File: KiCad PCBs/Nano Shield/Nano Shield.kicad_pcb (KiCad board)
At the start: 2 copper layers, 72.4 x 35.6 mm, 32 parts, among them J1 Conn_01x15_Female, J10 Screw_Terminal_01x02, J11 Screw_Terminal_01x02, J12 Screw_Terminal_01x02, J13 Screw_Terminal_01x02, J15 Screw_Terminal_01x02, J17 Screw_Terminal_01x02, J18 Screw_Terminal_01x02, J2 Conn_01x15_Female, J3 Screw_Terminal_01x02, J4 Screw_Terminal_01x02, J5 Screw_Terminal_01x02, J6 Screw_Terminal_01x02, J7 Screw_Terminal_01x02, J8 Screw_Terminal_01x02, J9 Screw_Terminal_01x02, SW1 SW_DIP_x02, SW2 SW_DIP_x02, U1 MAX487ESA+T, U2 AMS1117-5.0, U3 ULN2003A

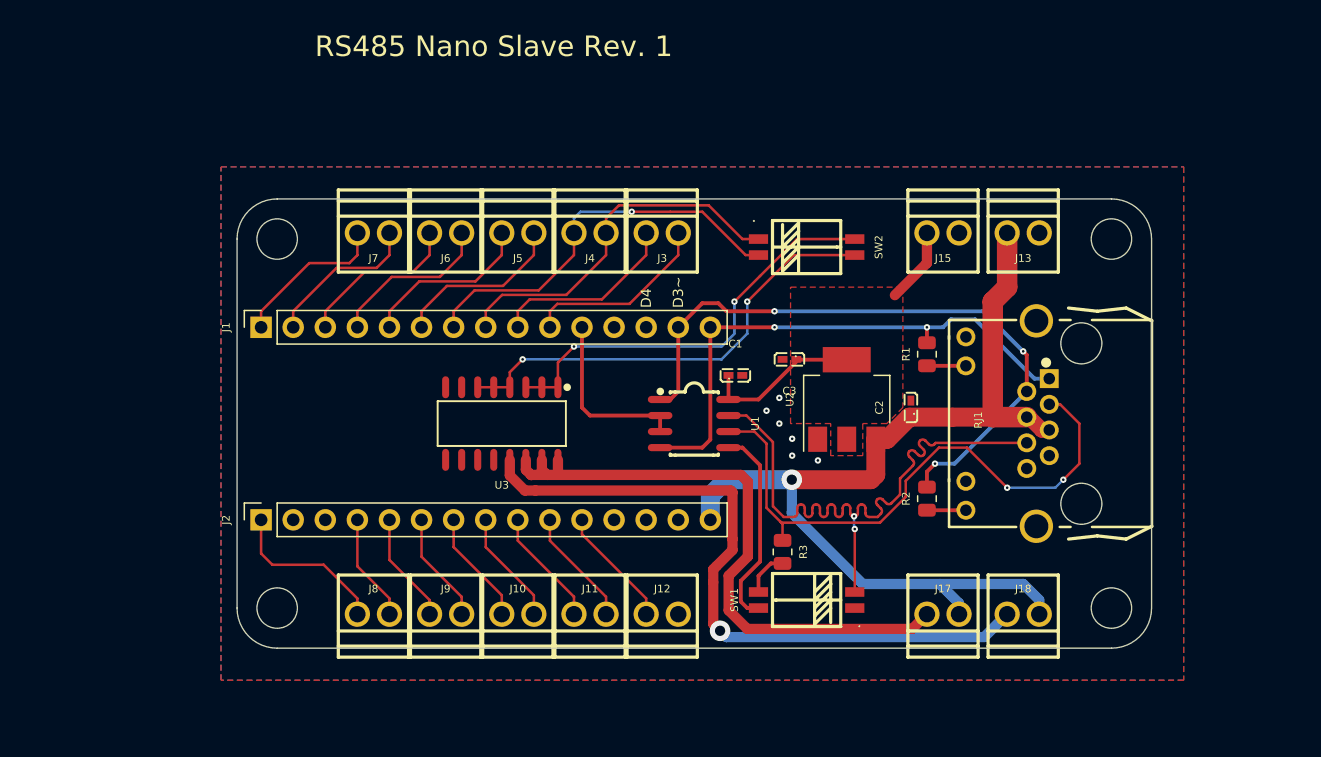
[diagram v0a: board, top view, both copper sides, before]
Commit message: Finished Nano Shield
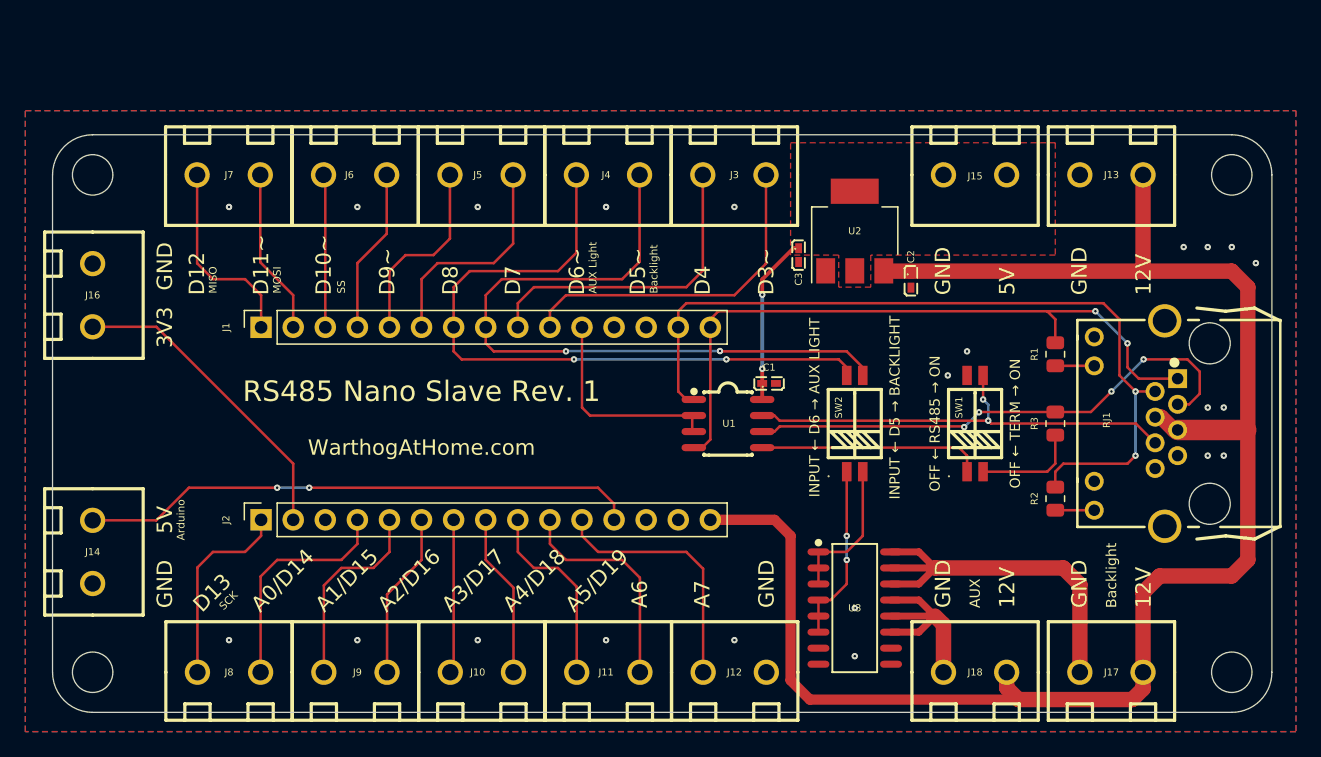
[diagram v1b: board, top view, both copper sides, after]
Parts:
- added J14: Screw_Terminal_01x02, A10 KiCad Libraries:CONN-TH_WJ126V-5.0-2P, F.Cu at (121.9, 111.8)
- added J16: Screw_Terminal_01x02, A10 KiCad Libraries:CONN-TH_WJ126V-5.0-2P, F.Cu at (121.9, 91.4)
- J10, J11, J12, J13, J15, J17, J18, J3, J4, J5, J6, J7, J8, J9: footprint A10 KiCad Libraries:CONN-TH_XY308-2.54-2P -> A10 KiCad Libraries:CONN-TH_WJ126V-5.0-2P
- moved U3 31.5 mm to (182.2, 116.2), turned to -90 degrees
- moved R3 23.9 mm to (198.1, 101.6)
- moved SW1 19.3 mm to (191.8, 101.6), turned to 0 degrees
- moved H1 15.5 mm to (121.9, 81.9)
- moved H3 15.5 mm to (121.9, 121.3)
- moved SW2 14.5 mm to (182.2, 101.6), turned to 0 degrees
- moved J17 14.1 mm to (202.6, 121.3), turned to 90 degrees
- moved U2 13.4 mm to (182.2, 86.4)
- moved J7 12.3 mm to (132.7, 81.9), turned to -90 degrees
- moved J8 12.3 mm to (132.7, 121.3), turned to 90 degrees
- moved H2 10.8 mm to (212.1, 81.9)
- moved H4 10.8 mm to (212.1, 121.3)
- moved R1 10.2 mm to (198.1, 96.1)
- moved R2 10.2 mm to (198.1, 107.5)
- moved RJ1 10.2 mm to (207.9, 101.6)
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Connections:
- J10 pad 1: A4/D18 -> A3/D17
- J10 pad 2: A3/D17 -> A4/D18
- J11 pad 1: A6 -> A5/D19
- J11 pad 2: A5/D19 -> A6
- J12 pad 1: GND -> A7
- J12 pad 2: A7 -> GND
- J17 pad 1: +12V -> BACKLIGHT_GND
- J17 pad 2: BACKLIGHT_GND -> +12V
- J18 pad 1: +12V -> AUX_GND
- J18 pad 2: AUX_GND -> +12V
- J3 pad 1: D4 -> D3~
- J3 pad 2: D3~ -> D4
- J4 pad 1: D6~/AUX_LIGHT -> D5~/BACKLIGHT
- J4 pad 2: D5~/BACKLIGHT -> D6~/AUX_LIGHT
- J5 pad 1: D8 -> D7
- J5 pad 2: D7 -> D8
- J6 pad 1: D10~/SS -> D9~
- J6 pad 2: D9~ -> D10~/SS
- J7 pad 1: D12/MISO -> D11~/MOSI
- J7 pad 2: D11~/MOSI -> D12/MISO
- J8 pad 1: A0/D14 -> D13/SCK
- J8 pad 2: D13/SCK -> A0/D14
- J9 pad 1: A2/D16 -> A1/D15
- J9 pad 2: A1/D15 -> A2/D16
- SW1 pad 1: GND -> RS485_GND
- SW1 pad 2: RS485- -> Net-(R3-Pad2)
- SW1 pad 3: Net-(R3-Pad2) -> RS485-
- SW1 pad 4: RS485_GND -> GND
- SW2 pad 1: D5~/BACKLIGHT -> AUX_BASE
- SW2 pad 2: D6~/AUX_LIGHT -> BACKLIGHT_BASE
- SW2 pad 3: AUX_BASE -> D5~/BACKLIGHT
- SW2 pad 4: BACKLIGHT_BASE -> D6~/AUX_LIGHT
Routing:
- net +12V: track 77.6 -> 132.9 mm, vias 1 -> 0
- net 5V_ARDUINO: track 0.00 -> 44.1 mm, vias 0 -> 2
- net AUX_GND: track 54.9 -> 16.2 mm, vias 1 -> 0
- net D5~/BACKLIGHT: track 29.1 -> 55.2 mm, vias 0 -> 2
- net +3V3: track 0.00 -> 24.8 mm
- net D6~/AUX_LIGHT: track 31.8 -> 54.4 mm, vias 1 -> 2
- net AUX_BASE: track 36.4 -> 14.2 mm
- net BACKLIGHT_BASE: track 33.5 -> 11.7 mm, vias 2 -> 0
- net BACKLIGHT_GND: track 49.1 -> 30.4 mm
- net RS485-: track 50.7 -> 35.8 mm
- net RXD: track 51.5 -> 64.5 mm, vias 3 -> 2
- net D3~: track 15.0 -> 27.0 mm
- net TXD: track 43.4 -> 54.4 mm
- net A7: track 9.57 -> 20.1 mm
- net D4: track 15.0 -> 25.2 mm
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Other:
- board size 72.4 x 35.6 mm -> 96.5 x 45.7 mm
- board text added: "BRRRRRRRRRRRRT"
- board text added: "WarthogAtHome.com"
